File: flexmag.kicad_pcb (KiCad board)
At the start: 2 copper layers, 181.7 x 16 mm, 7 parts, among them J1 Conn_01x06_Male, J2 Conn_01x06_Male, U1 AS5600-ASOM

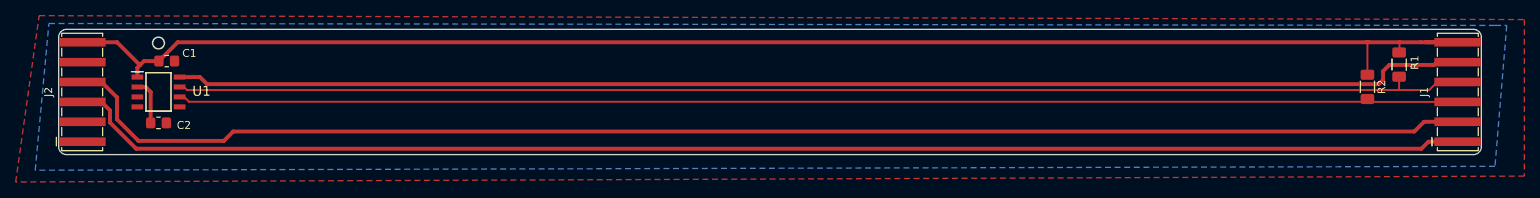
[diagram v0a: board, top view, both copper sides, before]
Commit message: Perfect is the enemy of done
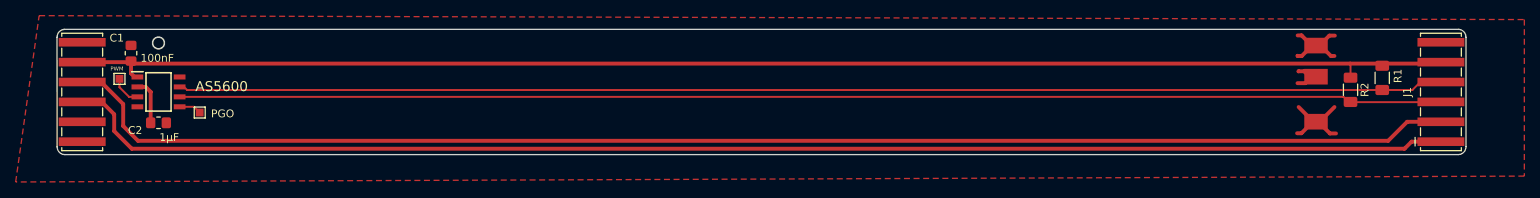
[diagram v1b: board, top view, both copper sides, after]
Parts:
- added REF**: TestPoint_Pad_1.0x1.0mm, TestPoint:TestPoint_Pad_1.0x1.0mm, F.Cu at (74.5, 50.9)
- added REF**: jmp, TestPoint:jmp, F.Cu at (217.1, 47.4)
- added REF**: TestPoint_Pad_1.0x1.0mm, TestPoint:TestPoint_Pad_1.0x1.0mm, F.Cu at (64.3, 46.6)
- moved C1 4.67 mm to (65.7, 43.3), turned to 90 degrees
- moved R1 2.75 mm to (225.6, 46.5)
- moved R2 2.19 mm to (221.5, 48.0)
- moved J1 2.16 mm to (233.1, 48.2)
- renumbered U1 to AS5600
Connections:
- J1 pad 5: GND -> +5V
- J1 pad 6: +5V -> GND
- J2 pad 5: GND -> +5V
- J2 pad 6: +5V -> GND
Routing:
- net GND: track 165.5 -> 29.2 mm
- net +5V: track 194.2 -> 178.3 mm
- net unconnected-(U1-Pad3): track 0.00 -> 3.87 mm
- net unconnected-(U1-Pad5): track 0.00 -> 2.87 mm
- net Net-(J1-Pad2): track 181.5 -> 179.4 mm
- net Net-(J1-Pad1): track 179.5 -> 177.7 mm
- net Net-(J1-Pad4): track 165.6 -> 164.0 mm
- net Net-(J1-Pad3): track 163.9 -> 162.5 mm
- removed copper zone on B.Cu, net +5V
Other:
- board size 181.7 x 16 mm -> 180 x 16 mm
- board text added: "PGO"
- board text added: "PWM"
